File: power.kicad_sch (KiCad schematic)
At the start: 30 parts, among them J1 GT-USB-7010ASV, P1 S2B-PH-SM4-TB, U1 BQ25185DLHR, U2 TPS73633DBVT, U3 TPS631000DRLR, U5 USBLC6-2SC6

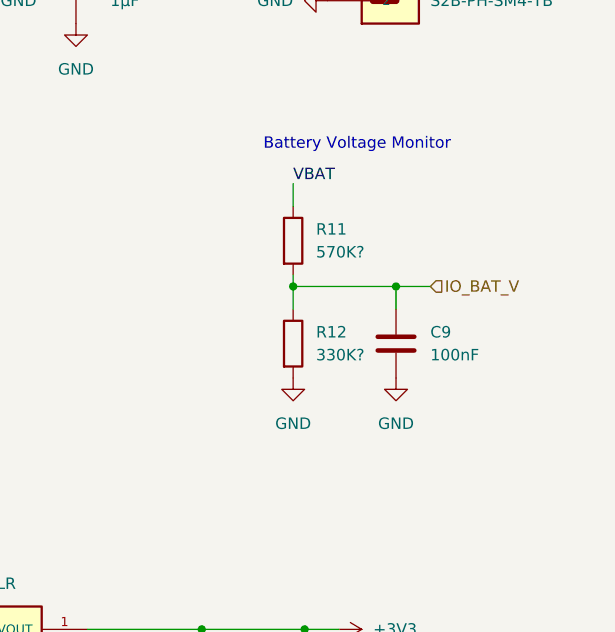
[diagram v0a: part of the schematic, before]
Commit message: fix sd card pullups
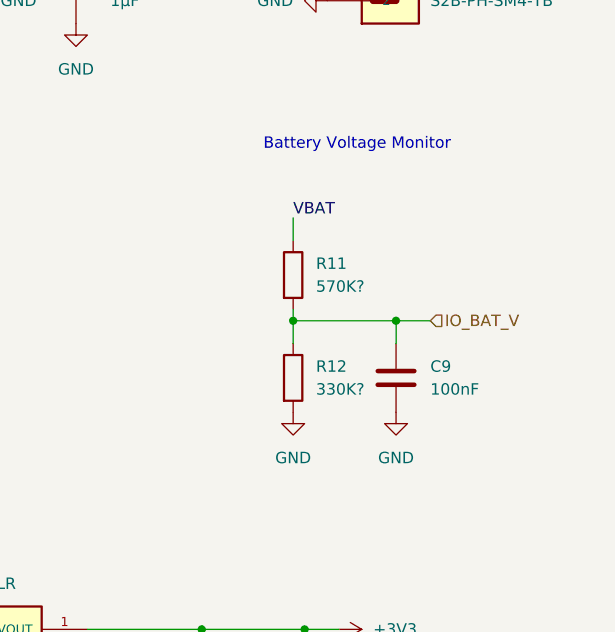
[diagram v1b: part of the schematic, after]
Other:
- moved on the sheet: C9, R11, R12
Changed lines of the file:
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@@
 	)
 	(junction
-		(at 247.65 77.47)
+		(at 247.65 81.28)
 		(diameter 0)
 		(color 0 0 0 0)
@@
 	)
 	(junction
-		(at 259.08 77.47)
+		(at 259.08 81.28)
 		(diameter 0)
 		(color 0 0 0 0)
@@
 	(wire
 		(pts
-			(xy 259.08 77.47) (xy 262.89 77.47)
+			(xy 259.08 81.28) (xy 262.89 81.28)
 		)
 		(stroke
@@
 	(wire
 		(pts
-			(xy 247.65 66.04) (xy 247.65 68.58)
+			(xy 247.65 69.85) (xy 247.65 72.39)
 		)
 		(stroke
@@
 	(wire
 		(pts
-			(xy 247.65 76.2) (xy 247.65 77.47)
+			(xy 247.65 80.01) (xy 247.65 81.28)
 		)
 		(stroke
@@
 	(wire
 		(pts
-			(xy 247.65 77.47) (xy 259.08 77.47)
+			(xy 247.65 81.28) (xy 259.08 81.28)
 		)
 		(stroke
@@
 	(wire
 		(pts
-			(xy 247.65 77.47) (xy 247.65 80.01)
+			(xy 247.65 81.28) (xy 247.65 83.82)
 		)
 		(stroke
@@
 	(wire
 		(pts
-			(xy 259.08 80.01) (xy 259.08 77.47)
+			(xy 259.08 83.82) (xy 259.08 81.28)
 		)
 		(stroke
@@
 		)
 	)
-	(label "USB_D+"
-		(at 74.93 53.34 0)
+	(label "VBAT"
+		(at 227.33 40.64 0)
 		(effects
 			(font
@@
 		)
 	)
-	(label "VBAT"
-		(at 227.33 40.64 0)
+	(label "USB_D+"
+		(at 74.93 53.34 0)
 		(effects
 			(font
@@
 	)
 	(label "VBAT"
-		(at 247.65 66.04 0)
+		(at 251.46 43.18 180)
 		(effects
 			(font
 				(size 1.27 1.27)
 			)
-			(justify left bottom)
+			(justify right bottom)
 		)
 	)
@@
 		)
 	)
-	(label "VBAT"
-		(at 251.46 43.18 180)
+	(label "USB_D-"
+		(at 39.37 55.88 180)
 		(effects
 			(font
@@
 		)
 	)
-	(label "USB_D-"
-		(at 39.37 55.88 180)
+	(label "VBAT"
+		(at 247.65 69.85 0)
 		(effects
 			(font
 				(size 1.27 1.27)
 			)
-			(justify right bottom)
+			(justify left bottom)
 		)
 	)
@@
 	(hierarchical_label "IO_BAT_V"
 		(shape input)
-		(at 262.89 77.47 0)
+		(at 262.89 81.28 0)
 		(effects
 			(font
@@
 	(symbol
 		(lib_id "power:GND")
-		(at 259.08 87.63 0)
+		(at 259.08 91.44 0)
 		(unit 1)
 		(body_style 1)
@@
 		(fields_autoplaced yes)
 		(property "Reference" "#PWR029"
-			(at 259.08 93.98 0)
+			(at 259.08 97.79 0)
 			(hide yes)
 			(show_name no)
@@
 		)
 		(property "Value" "GND"
-			(at 259.08 92.71 0)
+			(at 259.08 96.52 0)
 			(show_name no)
 			(do_not_autoplace no)
@@
 		)
 		(property "Footprint" ""
-			(at 259.08 87.63 0)
+			(at 259.08 91.44 0)
 			(hide yes)
 			(show_name no)
@@
 		)
 		(property "Datasheet" ""
-			(at 259.08 87.63 0)
+			(at 259.08 91.44 0)
 			(hide yes)
 			(show_name no)
@@
 		)
 		(property "Description" "Power symbol creates a global label with name \"GND\" , ground"
-			(at 259.08 87.63 0)
+			(at 259.08 91.44 0)
 			(hide yes)
 			(show_name no)
@@
 	(symbol
 		(lib_id "Device:R")
-		(at 247.65 72.39 0)
+		(at 247.65 76.2 0)
 		(unit 1)
 		(body_style 1)
@@
 		(fields_autoplaced yes)
 		(property "Reference" "R11"
-			(at 250.19 71.1199 0)
+			(at 250.19 74.9299 0)
 			(show_name no)
 			(do_not_autoplace no)
@@
 		)
 		(property "Value" "570K?"
-			(at 250.19 73.6599 0)
+			(at 250.19 77.4699 0)
 			(show_name no)
 			(do_not_autoplace no)
@@
 		)
 		(property "Footprint" "Resistor_SMD:R_0201_0603Metric"
-			(at 245.872 72.39 90)
+			(at 245.872 76.2 90)
 			(hide yes)
 			(show_name no)
@@
 		)
 		(property "Datasheet" ""
-			(at 247.65 72.39 0)
+			(at 247.65 76.2 0)
 			(hide yes)
 			(show_name no)
@@
 		)
 		(property "Description" "Resistor"
-			(at 247.65 72.39 0)
+			(at 247.65 76.2 0)
 			(hide yes)
 			(show_name no)
@@
 	(symbol
 		(lib_id "Device:R")
-		(at 247.65 83.82 0)
+		(at 247.65 87.63 0)
 		(unit 1)
 		(body_style 1)
@@
 		(fields_autoplaced yes)
 		(property "Reference" "R12"
-			(at 250.19 82.5499 0)
+			(at 250.19 86.3599 0)
 			(show_name no)
 			(do_not_autoplace no)
@@
 		)
 		(property "Value" "330K?"
-			(at 250.19 85.0899 0)
+			(at 250.19 88.8999 0)
 			(show_name no)
 			(do_not_autoplace no)
@@
 		)
 		(property "Footprint" "Resistor_SMD:R_0201_0603Metric"
-			(at 245.872 83.82 90)
+			(at 245.872 87.63 90)
 			(hide yes)
 			(show_name no)
@@
 		)
 		(property "Datasheet" ""
-			(at 247.65 83.82 0)
+			(at 247.65 87.63 0)
 			(hide yes)
 			(show_name no)
@@
 		)
 		(property "Description" "Resistor"
-			(at 247.65 83.82 0)
+			(at 247.65 87.63 0)
 			(hide yes)
 			(show_name no)
@@
 	(symbol
 		(lib_id "Device:C")
-		(at 259.08 83.82 0)
+		(at 259.08 87.63 0)
 		(unit 1)
 		(body_style 1)
@@
 		(fields_autoplaced yes)
 		(property "Reference" "C9"
-			(at 262.89 82.5499 0)
+			(at 262.89 86.3599 0)
 			(show_name no)
 			(do_not_autoplace no)
@@
 		)
 		(property "Value" "100nF"
-			(at 262.89 85.0899 0)
+			(at 262.89 88.8999 0)
 			(show_name no)
 			(do_not_autoplace no)
@@
 		)
 		(property "Footprint" "Capacitor_SMD:C_0201_0603Metric"
-			(at 260.0452 87.63 0)
+			(at 260.0452 91.44 0)
 			(hide yes)
 			(show_name no)
@@
 		)
 		(property "Datasheet" ""
-			(at 259.08 83.82 0)
+			(at 259.08 87.63 0)
 			(hide yes)
 			(show_name no)
@@
 		)
 		(property "Description" "Unpolarized capacitor"
-			(at 259.08 83.82 0)
+			(at 259.08 87.63 0)
 			(hide yes)
 			(show_name no)
@@
 	(symbol
 		(lib_id "power:GND")
-		(at 247.65 87.63 0)
+		(at 247.65 91.44 0)
 		(unit 1)
 		(body_style 1)
@@
 		(fields_autoplaced yes)
 		(property "Reference" "#PWR028"
-			(at 247.65 93.98 0)
+			(at 247.65 97.79 0)
 			(hide yes)
 			(show_name no)
@@
 		)
 		(property "Value" "GND"
-			(at 247.65 92.71 0)
+			(at 247.65 96.52 0)
 			(show_name no)
 			(do_not_autoplace no)
@@
 		)
 		(property "Footprint" ""
-			(at 247.65 87.63 0)
+			(at 247.65 91.44 0)
 			(hide yes)
 			(show_name no)
@@
 		)
 		(property "Datasheet" ""
-			(at 247.65 87.63 0)
+			(at 247.65 91.44 0)
 			(hide yes)
 			(show_name no)
@@
 		)
 		(property "Description" "Power symbol creates a global label with name \"GND\" , ground"
-			(at 247.65 87.63 0)
+			(at 247.65 91.44 0)
 			(hide yes)
 			(show_name no)
